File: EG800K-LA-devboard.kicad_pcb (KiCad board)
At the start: 4 copper layers, 35 x 35 mm, 49 parts, among them J1 U.FL-R-SMT_10_, J2 MICROQTJ, J5 Conn_01x08_Pin, Q1 DTC143ZUAT106, Q2 DTC143ZUAT106, Q4 DTC143ZUAT106, Q5 DTC143ZUAT106, Q6 BSS138, Q7 BSS138, Q8 BSS138, U4 EG800KEULC-I03-SNNSA

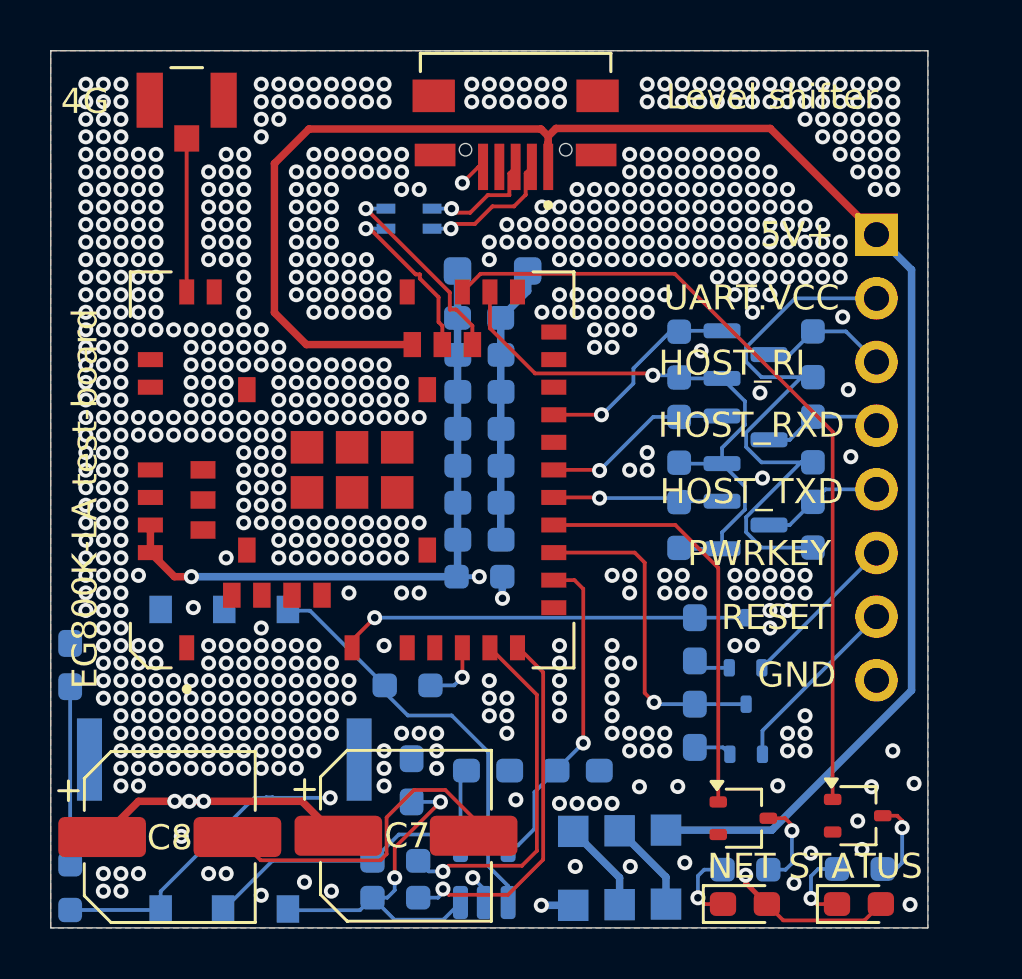
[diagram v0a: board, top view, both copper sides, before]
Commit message: version final
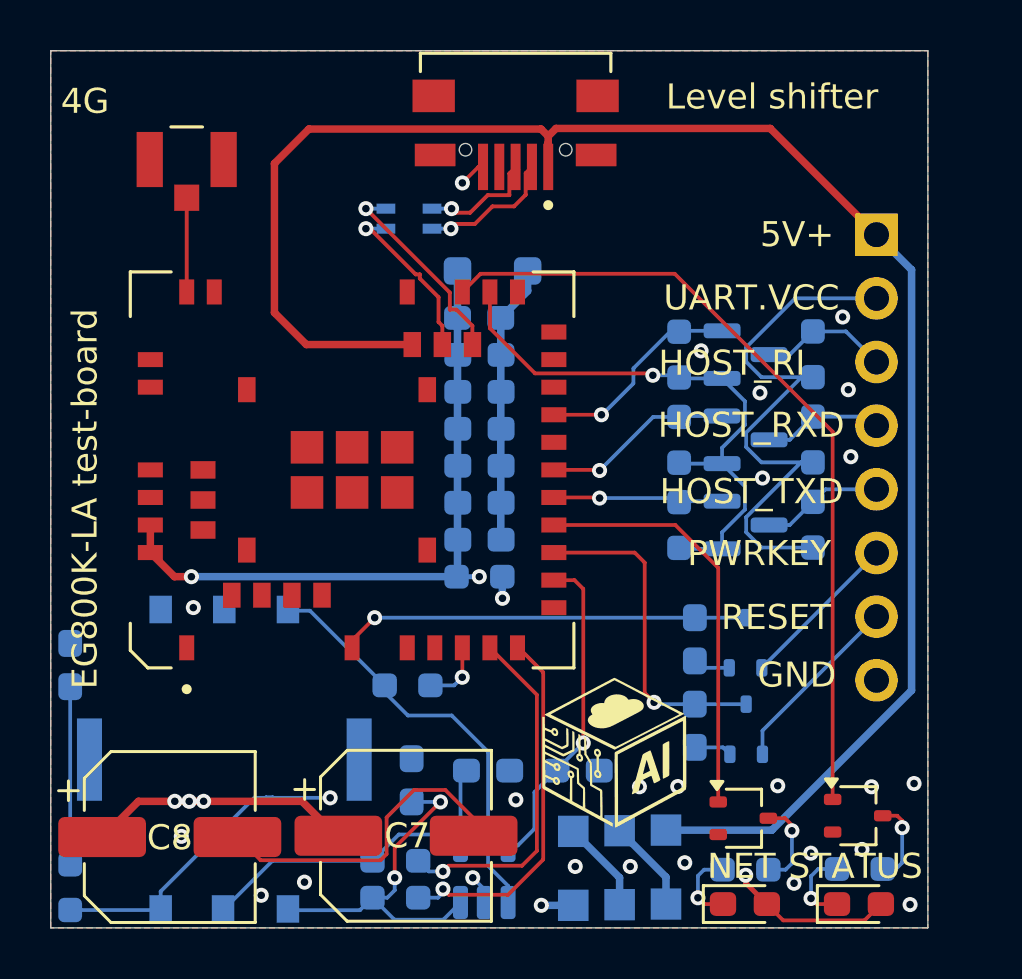
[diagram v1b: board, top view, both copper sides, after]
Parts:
- removed the G*** at (151.1, 70.5)
- added G***: LOGO, Images:LOGOv3.4, F.Cu at (166.6, 88.8)
- moved J1 2.36 mm to (149.5, 65.0)
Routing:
- net /RF_ANT: track 6.12 -> 3.76 mm
- net GND: vias 729 -> 25
